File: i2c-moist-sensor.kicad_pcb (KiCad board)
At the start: 2 copper layers, 18 x 149 mm, 25 parts, among them IC1 ATTINY441-SSU, P1 CONN_02X03, X1 16MHz

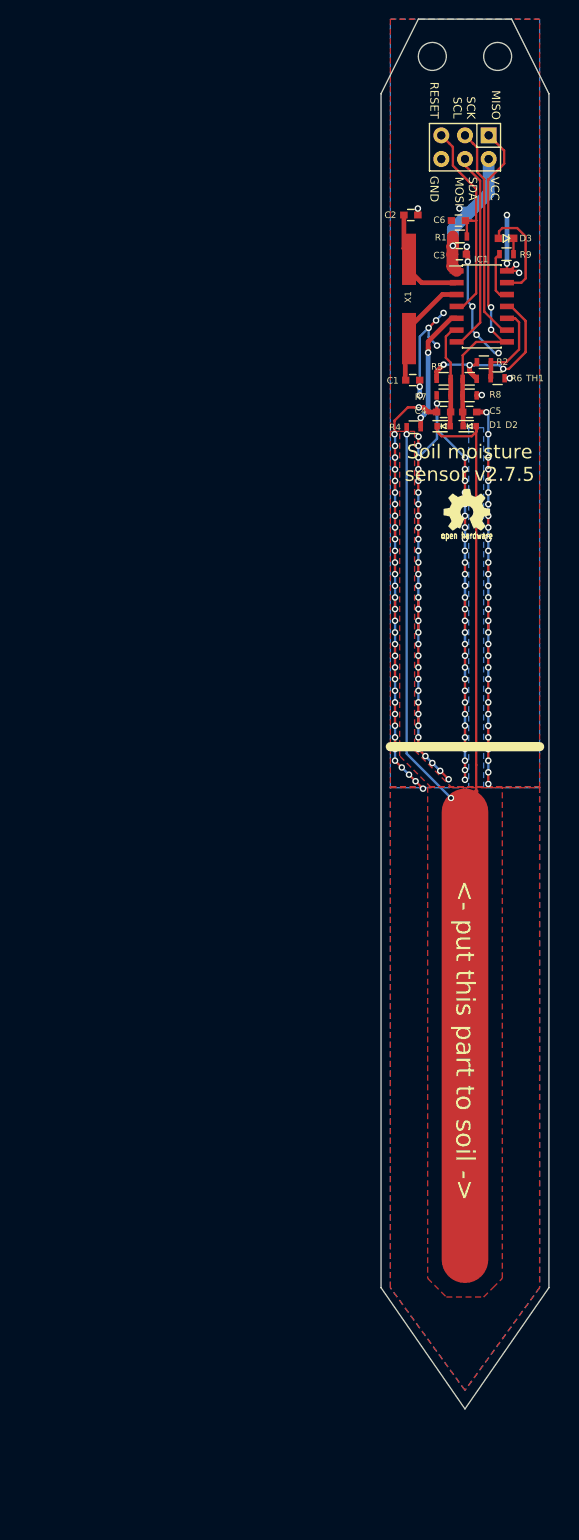
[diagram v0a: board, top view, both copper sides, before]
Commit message: SPBTLE version 1.0 - HW
Only hardware changes
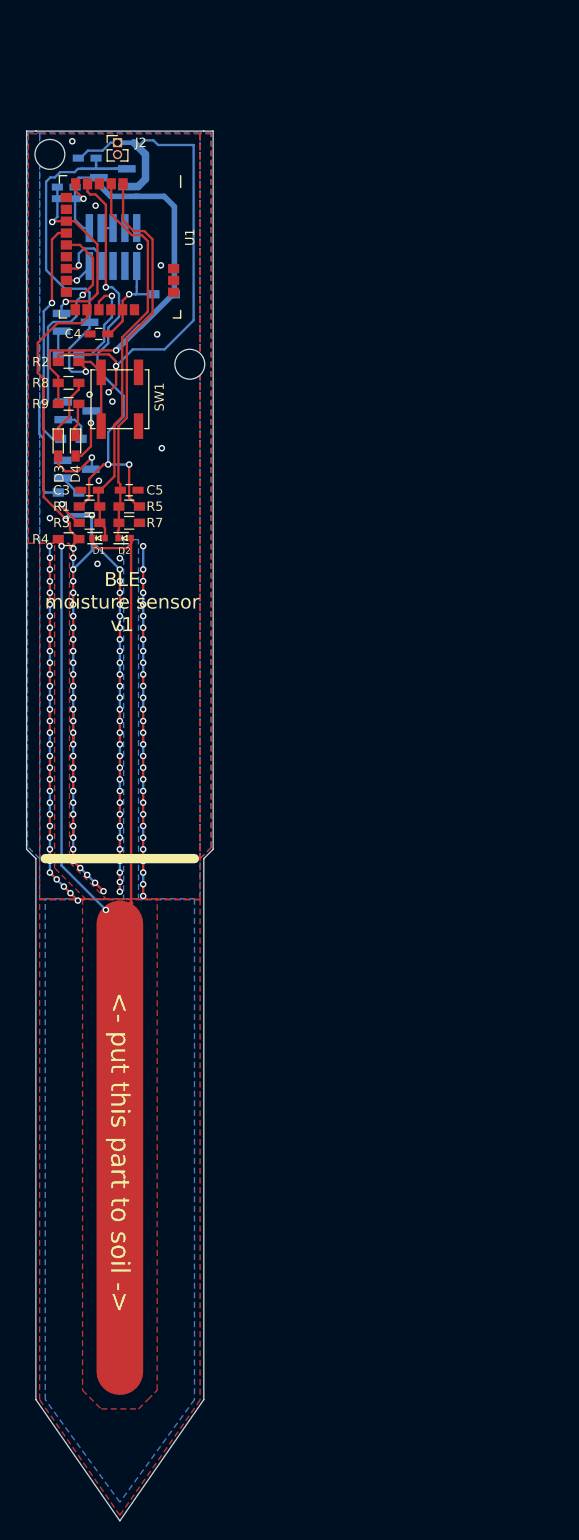
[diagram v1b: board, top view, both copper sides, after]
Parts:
- removed C2: 33pp, Capacitors_SMD:C_0603
- removed G***: LOGO, w_logo:Logo_silk_OSHW_6x6mm
- removed G***: LOGO, chirp_logo:ziogas
- removed IC1: ATTINY441-SSU, Housings_SOIC:SOIC-14_3.9x8.7mm_Pitch1.27mm
- removed P1: CONN_02X03, Pin_Headers:Pin_Header_Straight_2x03
- removed the REF** at (91.5, 17.0)
- removed the REF** at (98.5, 17.0)
- removed TH1: NCP18XH103F03RB, Resistors_SMD:R_0603
- removed X1: 16MHz, Crystals:Crystal_HC49-SD_SMD
- added C7: 1u, Capacitors_SMD:C_0603_HandSoldering, B.Cu at (52.2, 32.2)
- added D4: LED, LEDs:LED_0603_HandSoldering, F.Cu at (53.2, 58.7)
- added J1: Conn_02x05_Odd_Even, SBenoit:50mils_JTAG, B.Cu at (57.3, 37.4)
- added J2: Conn_01x02, Pin_Headers:Pin_Header_Straight_1x02_Pitch1.27mm, F.Cu at (57.8, 26.2)
- added Q1: BSS83P, TO_SOT_Packages_SMD:SOT-23_Handsoldering, B.Cu at (57.2, 30.0)
- added Q2: RUC002N05HZGT116CT, TO_SOT_Packages_SMD:SOT-23_Handsoldering, B.Cu at (53.2, 45.5)
- added Q3: RUC002N05HZGT116CT, TO_SOT_Packages_SMD:SOT-23_Handsoldering, B.Cu at (53.4, 61.2)
- added Q4: RUC002N05HZGT116CT, TO_SOT_Packages_SMD:SOT-23_Handsoldering, B.Cu at (53.4, 55.0)
- added R10: 100, Resistors_SMD:R_0603_HandSoldering, B.Cu at (52.5, 49.0)
- added R11: 100, Resistors_SMD:R_0603_HandSoldering, B.Cu at (52.5, 63.8)
- added R12: 100, Resistors_SMD:R_0603_HandSoldering, B.Cu at (52.8, 58.0)
- added R3: 1M, Resistors_SMD:R_0603_HandSoldering, F.Cu at (54.8, 67.0)
- added REF**: MountingHole_3.2mm_M3, Mounting_Holes:MountingHole_3.2mm_M3, F.Cu at (50.5, 27.5)
- added REF**: MountingHole_3.2mm_M3, Mounting_Holes:MountingHole_3.2mm_M3, F.Cu at (65.5, 50.0)
- added SW1: SW_Push, Buttons_Switches_SMD:SW_SPST_EVPBF, F.Cu at (58.0, 53.8)
- added U1: SPBTLE-1S, SBenoit:SPBTLE-1s, F.Cu at (58.8, 36.4)
- C1: value 33p -> 330n; footprint Capacitors_SMD:C_0603 -> Capacitors_SMD:C_0603_HandSoldering; moved to B.Cu
- C3: value 1u -> 1n; footprint Capacitors_SMD:C_0603 -> Capacitors_SMD:C_0603_HandSoldering
- C4: value 1n -> 10n; footprint Capacitors_SMD:C_0603 -> Capacitors_SMD:C_0603_HandSoldering
- C5: footprint Capacitors_SMD:C_0603 -> Capacitors_SMD:C_0603_HandSoldering
- C6: value 1u -> 100n; footprint Capacitors_SMD:C_0603 -> Capacitors_SMD:C_0603_HandSoldering; moved to B.Cu
- D3: footprint LEDs:LED-0603 -> LEDs:LED_0603_HandSoldering
- R1: value 10k -> 1M; footprint Resistors_SMD:R_0603 -> Resistors_SMD:R_0603_HandSoldering
- R2: value 10k 0.1% -> 1M; footprint Resistors_SMD:R_0603 -> Resistors_SMD:R_0603_HandSoldering
- R4, R5, R7, R9: footprint Resistors_SMD:R_0603 -> Resistors_SMD:R_0603_HandSoldering
- R6: value 1M -> 47k; footprint Resistors_SMD:R_0603 -> Resistors_SMD:R_0603_HandSoldering; moved to B.Cu
- R8: value 1M -> 330; footprint Resistors_SMD:R_0603 -> Resistors_SMD:R_0603_HandSoldering
- moved D3 52.9 mm to (51.4, 58.7)
- moved R9 49.6 mm to (52.5, 54.2)
- moved R1 49.1 mm to (54.8, 65.2)
- moved C3 47.0 mm to (54.8, 63.5), turned to 180 degrees
- moved R2 44.5 mm to (52.5, 49.8)
- moved R8 43.0 mm to (52.5, 52.0)
- moved C1 42.2 mm to (54.5, 27.9)
- moved C6 42.2 mm to (52.2, 31.0), turned to 0 degrees
- moved D2 38.9 mm to (58.5, 68.6)
- moved R4 38.9 mm to (52.5, 68.8)
- moved D1 38.9 mm to (55.7, 68.6)
- moved C4 37.9 mm to (55.8, 46.8)
- moved C5 37.5 mm to (59.0, 63.5)
- moved R5 36.4 mm to (59.0, 65.2), turned to 0 degrees
- moved R7 36.4 mm to (59.0, 67.0), turned to 180 degrees
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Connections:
- C1 pad 1: Net-(C1-Pad1) -> +3V0
- C1 pad 2: GND -> Net-(C1-Pad2)
- C3 pad 1: VCC -> /SENSE_LOW
- C4 pad 1: /SENSE_LOW -> /RESET
- C5 pad 1: /MISO/SENSE_HIGH -> /SENSE_HIGH
- C6 pad 1: /RESET -> GND
- C6 pad 2: GND -> VCC
- D2 pad 2: /MISO/SENSE_HIGH -> /SENSE_HIGH
- R1 pad 1: /RESET -> /SENSE_LOW
- R1 pad 2: VCC -> /POWER
- R2 pad 1: Net-(IC1-Pad11) -> +3V0
- R2 pad 2: /THERMISTOR -> Net-(C1-Pad2)
- R5 pad 1: /SENSE_LOW -> /SENSE_HIGH
- R5 pad 2: Net-(IC1-Pad11) -> /POWER
- R6 pad 1: /MISO/SENSE_HIGH -> /RESET
- R6 pad 2: Net-(IC1-Pad11) -> VCC
- R7 pad 2: /SENSE_LOW -> /SENSE_HIGH
- R8 pad 1: GND -> Net-(D3-Pad1)
- R8 pad 2: /MISO/SENSE_HIGH -> VCC
- R9 pad 1: Net-(D3-Pad2) -> Net-(D4-Pad1)
- R9 pad 2: Net-(IC1-Pad12) -> VCC
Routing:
- net GND: track 223.8 -> 108.4 mm, vias 145 -> 78
- net /EXCITATION: track 13.6 -> 127.7 mm, vias 2 -> 63
- net +3V0: track 0.00 -> 59.7 mm, vias 0 -> 2
- net Net-(C1-Pad2): track 0.00 -> 53.4 mm, vias 0 -> 1
- net /POWER: track 0.00 -> 48.5 mm, vias 0 -> 3
- net /SENSE_HIGH: track 0.00 -> 41.7 mm
- net /MISO/SENSE_HIGH: track 38.1 -> 0.00 mm, vias 2 -> 0
- net VCC: track 16.5 -> 52.9 mm
- net /SENSE_LOW: track 11.5 -> 42.9 mm
- net /LED1: track 0.00 -> 31.2 mm, vias 0 -> 1
- net /LED2: track 0.00 -> 27.4 mm, vias 0 -> 1
- net /SCK/SCL: track 23.0 -> 0.00 mm
- net /MOSI/SDA: track 21.7 -> 0.00 mm
- net Net-(IC1-Pad11): track 20.2 -> 0.00 mm, vias 3 -> 0
- net /RESET: track 24.1 -> 11.1 mm, vias 0 -> 1
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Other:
- board size 18 x 149 mm -> 20 x 149 mm
- rule trace_min: 0.254 -> 0.13
- rule via_min_drill: 0.4 -> 0.2
- rule via_min_size: 0.7 -> 0.45
- board text added: "BLE moisture sensor v1"
- board text added: "Originally from : Catnip Electronics http://wemakethings.net/chirp mic@wemakethings.net Modified by : Simon Benoit Gitbuh : Eriobis spiky1987@hotmail.com"
- board text removed: "Catnip Electronics http://wemakethings.net/chirp mic@wemakethings.net"
- board text removed: "GND"
- board text removed: "MISO"
- board text removed: "RESET"
- board text removed: "SCK SCL"
- board text removed: "SDA MOSI"
- board text removed: "Soil moisture sensor v2.7.5"
- board text removed: "VCC"
